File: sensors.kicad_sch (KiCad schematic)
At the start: 12 parts

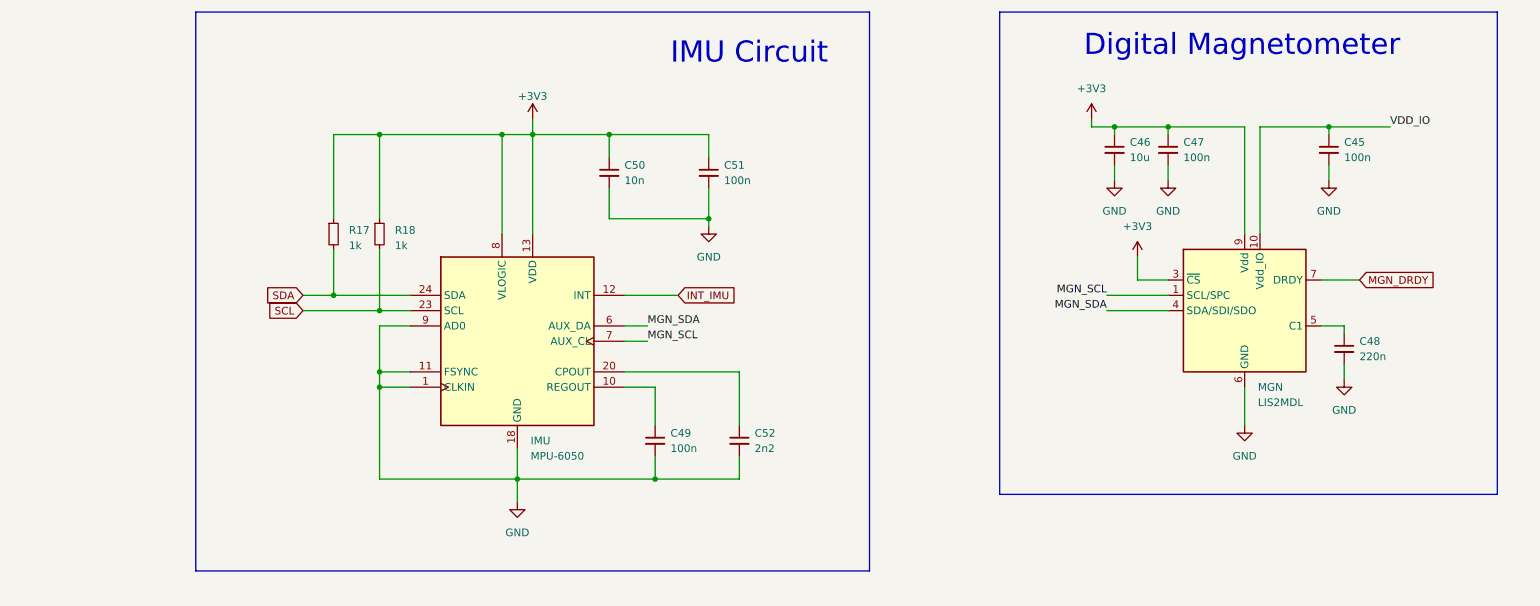
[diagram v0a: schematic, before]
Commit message: checkpoint for backup
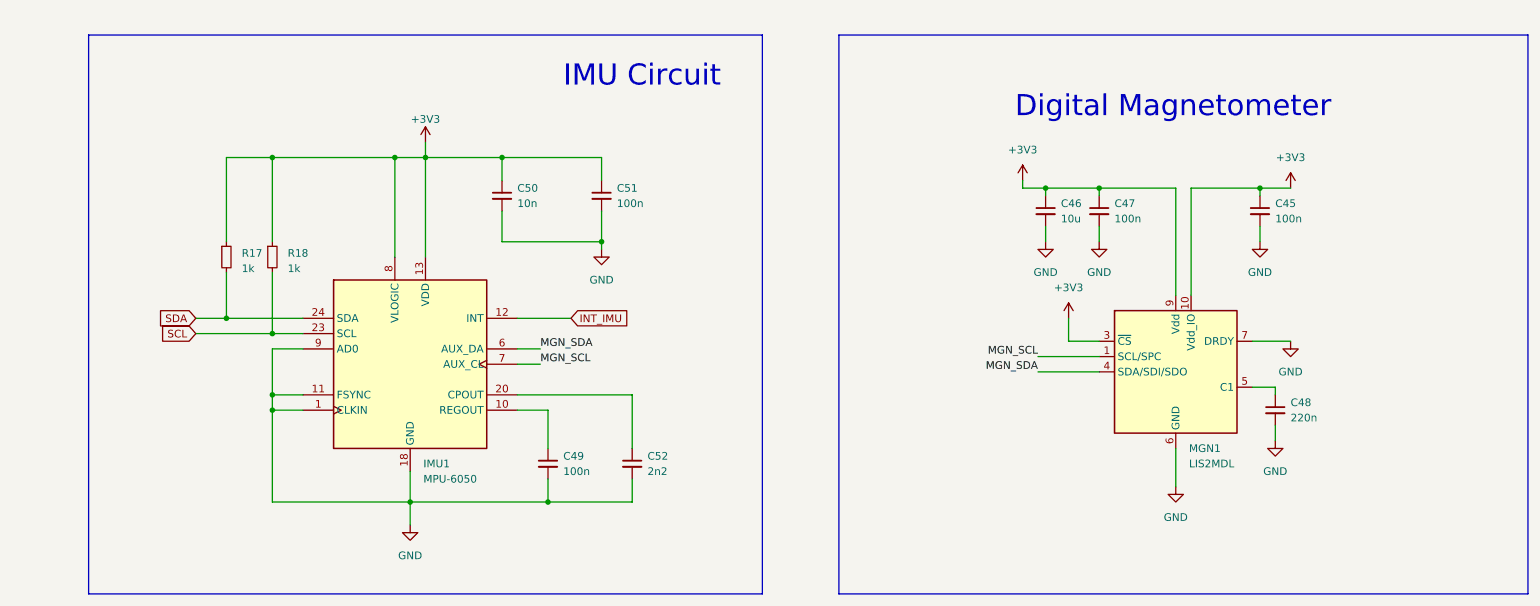
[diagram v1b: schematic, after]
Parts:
- renumbered IMU to IMU1, MGN to MGN1
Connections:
- net MGN_DRDY is gone; now on net GND: MGN1.7 (DRDY)
- net VDD_IO is gone; now on net +3V3: C45.1, MGN1.10 (Vdd_IO)
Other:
- moved on the sheet: C45, C46, C47, C48, C49, C50, C51, C52, IMU1, MGN1, R17, R18

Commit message: pcb updates & improvements
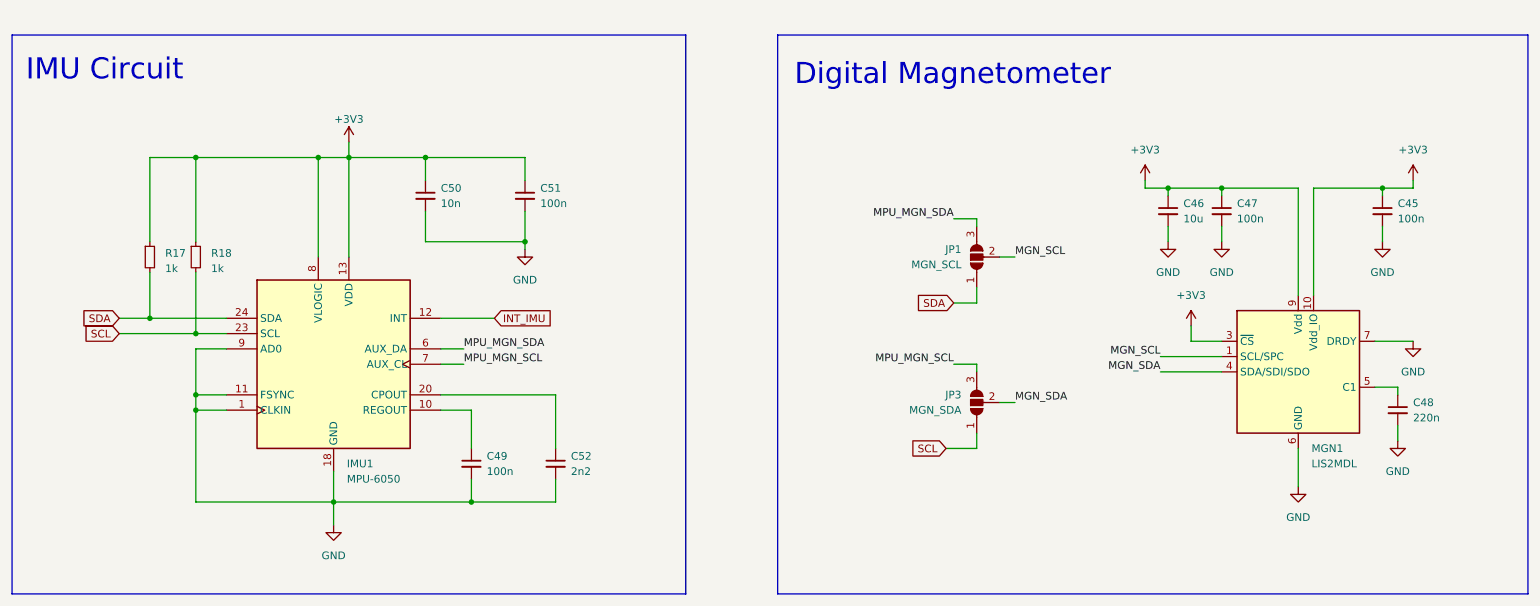
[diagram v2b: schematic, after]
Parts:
- added JP1: MGN_SCL, Jumper:SolderJumper-3_P2.0mm_Open_TrianglePad1.0x1.5mm, symbol Jumper:SolderJumper_3_Open
- added JP3: MGN_SDA, Jumper:SolderJumper-3_P2.0mm_Open_TrianglePad1.0x1.5mm, symbol Jumper:SolderJumper_3_Open
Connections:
- net MGN_SCL: now also JP1.2 (C); no longer IMU1.7 (AUX_CL)
- net MGN_SDA: now also JP3.2 (C); no longer IMU1.6 (AUX_DA)
- net SCL: now also JP3.1 (A)
- net SDA: now also JP1.1 (A)
- new net MPU_MGN_SCL: IMU1.7 (AUX_CL), JP3.3 (B)
- new net MPU_MGN_SDA: IMU1.6 (AUX_DA), JP1.3 (B)
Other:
- moved on the sheet: C45, C46, C47, C48, C49, C50, C51, C52, IMU1, MGN1, R17, R18
